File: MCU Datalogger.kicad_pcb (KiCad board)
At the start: 2 copper layers, 29 parts, among them J1 Conn_01x04_Male, J2 Conn_01x09_Male, J3 Conn_01x04_Male, J4 Conn_02x03_Odd_Even, U1 24LC1025, U2 DS1337S+, U3 24LC1025, U4 ATMEGA328P-AU, Y1 32.768 KHz, Y2 16 MHz

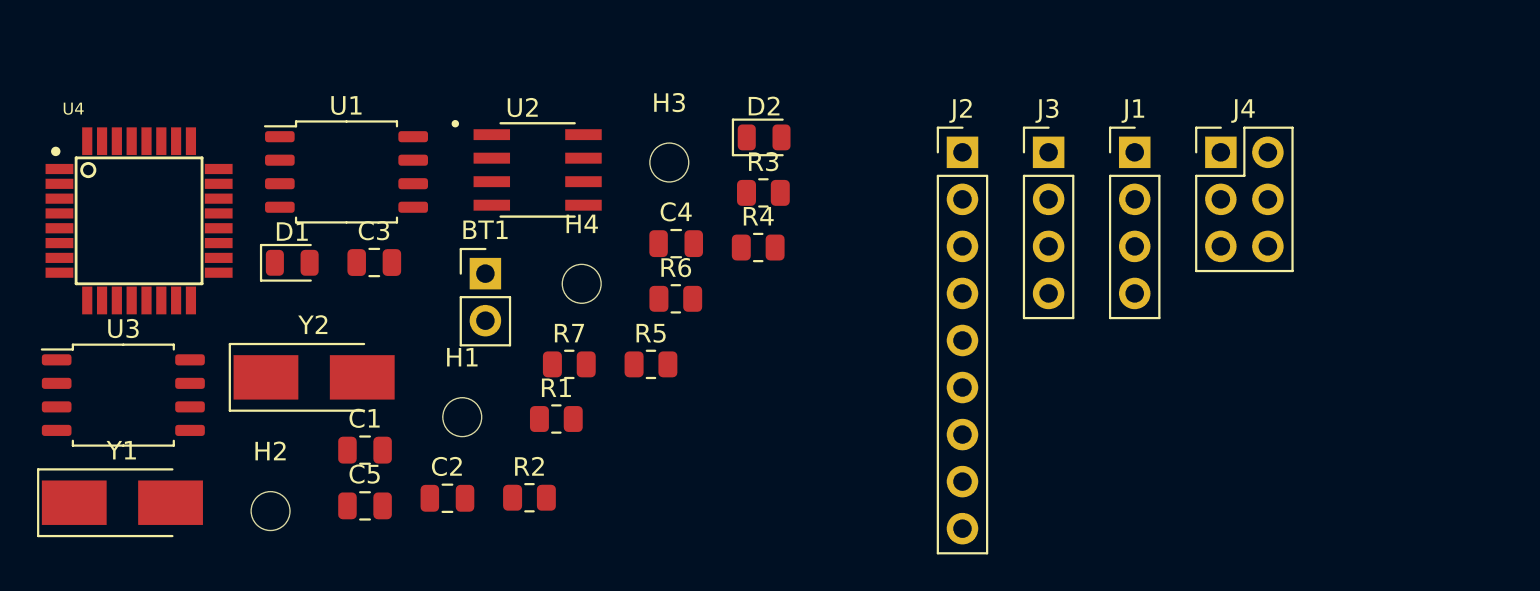
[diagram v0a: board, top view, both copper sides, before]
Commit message: Setup Pcbnew.
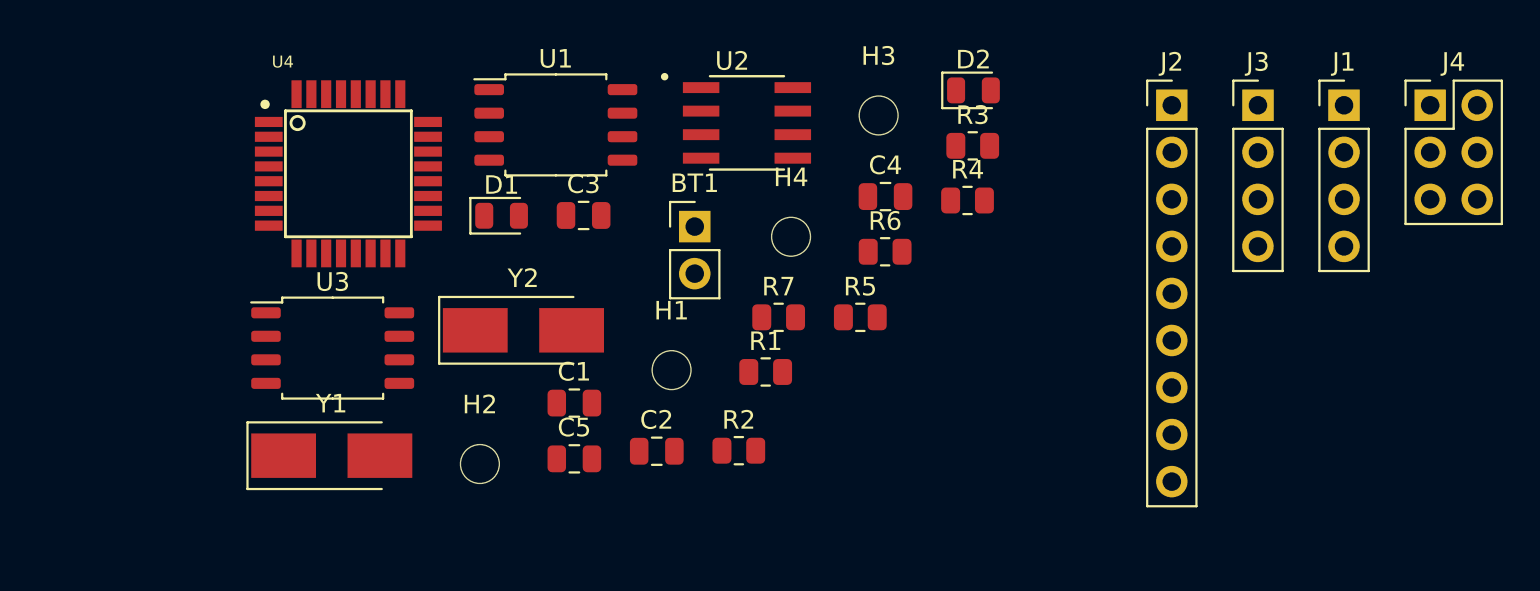
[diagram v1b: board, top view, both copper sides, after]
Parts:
- moved BT1 11.6 mm to (220.3, 86.9)
- moved C1 11.6 mm to (213.8, 96.4)
- moved C3 11.6 mm to (214.3, 86.3)
- moved H1 11.6 mm to (219.1, 94.6)
- moved H3 11.6 mm to (230.3, 80.9)
- moved J1 11.6 mm to (255.4, 80.3)
- moved J2 11.6 mm to (246.1, 80.3)
- moved J3 11.6 mm to (250.8, 80.3)
- moved J4 11.6 mm to (260.1, 80.3)
- moved R3 11.6 mm to (235.4, 82.5)
- moved R4 11.6 mm to (235.1, 85.5)
- moved R5 11.6 mm to (229.3, 91.8)
- moved R6 11.6 mm to (230.6, 88.2)
- moved R7 11.6 mm to (224.9, 91.8)
- moved U1 11.6 mm to (212.8, 81.4)
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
